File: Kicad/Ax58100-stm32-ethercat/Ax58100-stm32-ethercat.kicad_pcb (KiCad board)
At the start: 4 copper layers, 94.5 x 59.2 mm, 133 parts, among them J1 Conn_01x06_Pin, J10 Conn_01x02_Pin, J11 Stepper 2, J12 Serial usart1, J13 Stepper 1, J14 I2C bus2, J2 Encoder 1, J3 Conn_01x06_Pin, J4 Encoder 2, J5 Conn_01x06_Pin, J6 Encoder 4, J7 DAC1, J8 Encoder 3, J9 STLINK, SW1 SW PB, U1 AMS1117-1.2, U2 AX58100, U3 24LC32A, U4 STM32F407VGT6, U5 AMS1117-3.3, Y1 NXK25.000AE12F-KAB6-12, Y2 8 MHz

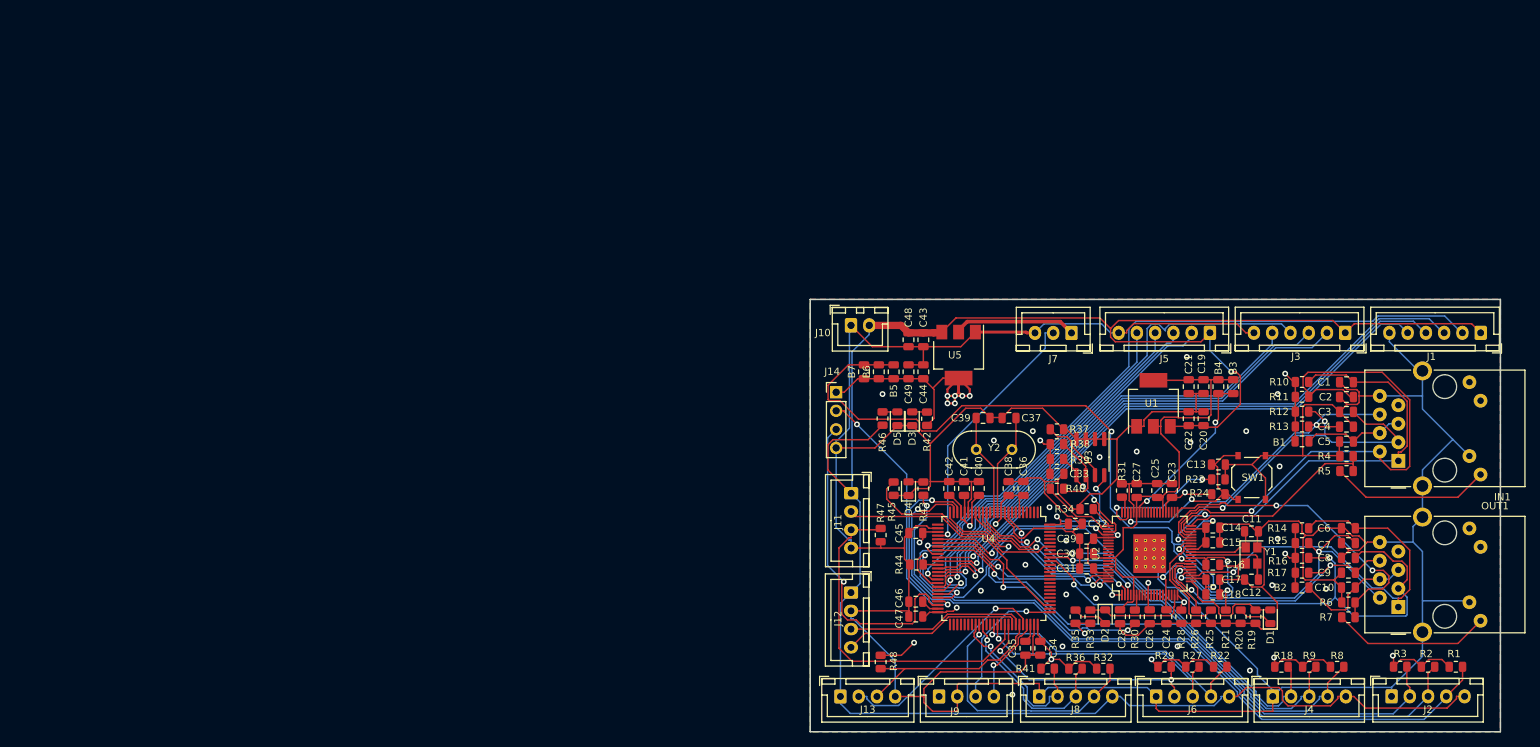
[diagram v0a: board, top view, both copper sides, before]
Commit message: First component placement
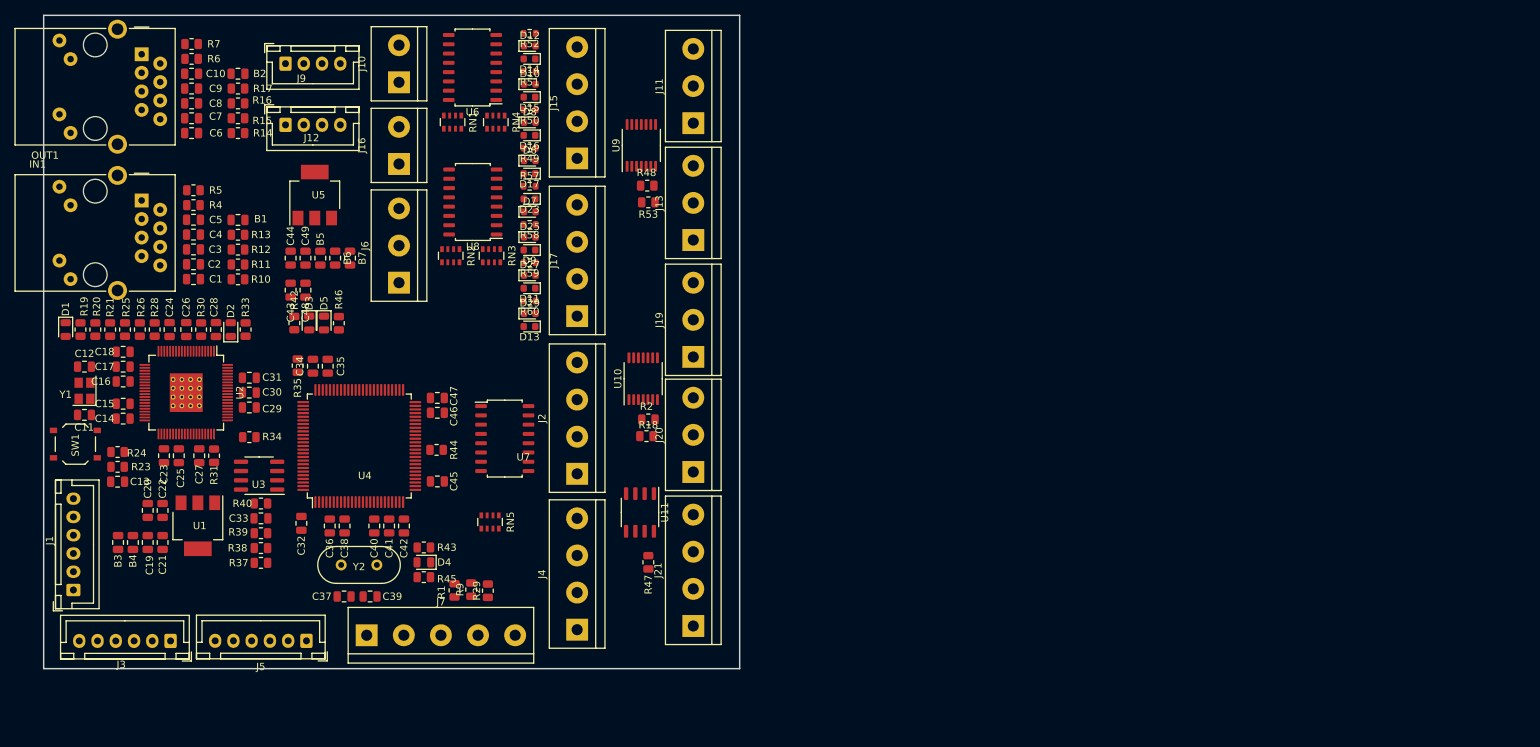
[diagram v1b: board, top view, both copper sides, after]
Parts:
- removed J14: I2C bus2, Connector_PinHeader_2.54mm:PinHeader_1x04_P2.54mm_Vertical
- removed J8: Encoder 3, Connector_JST:JST_XH_B5B-XH-A_1x05_P2.50mm_Vertical
- removed R22, R27, R3, R32, R36, R41, R8: 1k, Resistor_SMD:R_0805_2012Metric
- added D10: Yellow led, LED_SMD:LED_0603_1608Metric, F.Cu at (100.6, 34.3)
- added D11: Red led, LED_SMD:LED_0603_1608Metric, F.Cu at (100.5, 62.2)
- added D12: Yellow led, LED_SMD:LED_0603_1608Metric, F.Cu at (100.6, 29.1)
- added D13: Red led, LED_SMD:LED_0603_1608Metric, F.Cu at (100.5, 67.5)
- added D14: Red led, LED_SMD:LED_0603_1608Metric, F.Cu at (100.5, 30.8)
- added D15: Red led, LED_SMD:LED_0603_1608Metric, F.Cu at (100.5, 36.1)
- added D16: Red led, LED_SMD:LED_0603_1608Metric, F.Cu at (100.5, 41.3)
- added D17: Red led, LED_SMD:LED_0603_1608Metric, F.Cu at (100.5, 46.5)
- added D23: Yellow led, LED_SMD:LED_0603_1608Metric, F.Cu at (100.5, 50.0)
- added D25: Yellow led, LED_SMD:LED_0603_1608Metric, F.Cu at (100.6, 55.2)
- added D27: Yellow led, LED_SMD:LED_0603_1608Metric, F.Cu at (100.6, 60.5)
- added D29: Yellow led, LED_SMD:LED_0603_1608Metric, F.Cu at (100.6, 65.7)
- added D6: Yellow led, LED_SMD:LED_0603_1608Metric, F.Cu at (100.6, 44.8)
- added D7: Red led, LED_SMD:LED_0603_1608Metric, F.Cu at (100.6, 51.8)
- added D8: Yellow led, LED_SMD:LED_0603_1608Metric, F.Cu at (100.6, 39.5)
- added D9: Red led, LED_SMD:LED_0603_1608Metric, F.Cu at (100.5, 57.0)
- added J15: In1-4, TerminalBlock:TerminalBlock_bornier-4_P5.08mm, F.Cu at (107.0, 44.5)
- added J16: 24V Field, TerminalBlock:TerminalBlock_bornier-2_P5.08mm, F.Cu at (82.7, 45.2)
- added J17: In5-8, TerminalBlock:TerminalBlock_bornier-4_P5.08mm, F.Cu at (107.0, 66.0)
- added J19: Step3, TerminalBlock:TerminalBlock_bornier-3_P5.08mm, F.Cu at (122.9, 71.6)
- added J20: Step4, TerminalBlock:TerminalBlock_bornier-3_P5.08mm, F.Cu at (122.9, 87.4)
- added J21: THCAD, TerminalBlock:TerminalBlock_bornier-4_P5.08mm, F.Cu at (122.9, 108.5)
- added R49: 1k, Resistor_SMD:R_0603_1608Metric, F.Cu at (100.5, 43.0)
- added R50: 1k, Resistor_SMD:R_0603_1608Metric, F.Cu at (100.5, 37.8)
- added R51: 1k, Resistor_SMD:R_0603_1608Metric, F.Cu at (100.5, 32.6)
- added R52: 1k, Resistor_SMD:R_0603_1608Metric, F.Cu at (100.5, 27.3)
- added R53: 4.7k, Resistor_SMD:R_0805_2012Metric, F.Cu at (116.8, 50.5)
- added R57: 1k, Resistor_SMD:R_0603_1608Metric, F.Cu at (100.5, 48.3)
- added R58: 1k, Resistor_SMD:R_0603_1608Metric, F.Cu at (100.5, 53.5)
- added R59: 1k, Resistor_SMD:R_0603_1608Metric, F.Cu at (100.5, 58.7)
- added R60: 1k, Resistor_SMD:R_0603_1608Metric, F.Cu at (100.5, 64.0)
- added RN1: 40k, Resistor_SMD:R_Array_Convex_4x0603, F.Cu at (90.0, 39.5)
- added RN2: 40k, Resistor_SMD:R_Array_Convex_4x0603, F.Cu at (89.7, 57.8)
- added RN3: 1k, Resistor_SMD:R_Array_Convex_4x0603, F.Cu at (95.3, 57.8)
- added RN4: 1k, Resistor_SMD:R_Array_Convex_4x0603, F.Cu at (95.9, 39.5)
- added RN5: 330, Resistor_SMD:R_Array_Convex_4x0603, F.Cu at (95.1, 94.2)
- added U10: TXB0104PW, Package_SO:TSSOP-14_4.4x5mm_P0.65mm, F.Cu at (116.1, 74.6)
- added U11: MAX3485CSA/ESA, Package_SO:SO-8_3.9x4.9mm_P1.27mm, F.Cu at (115.6, 92.9)
- added U6: TLP292-4, Package_SO:SOIC-16_4.55x10.3mm_P1.27mm, F.Cu at (92.7, 32.0)
- added U7: TLP291-4, Package_SO:SOIC-16_4.55x10.3mm_P1.27mm, F.Cu at (97.1, 82.8)
- added U8: TLP292-4, Package_SO:SOIC-16_4.55x10.3mm_P1.27mm, F.Cu at (92.8, 50.4)
- added U9: TXB0104PW, Package_SO:TSSOP-14_4.4x5mm_P0.65mm, F.Cu at (115.8, 42.7)
- J1: value Conn_01x06_Pin -> Out_opt
- J10: value Conn_01x02_Pin -> 5V Power IN; footprint Connector_JST:JST_XH_B2B-XH-A_1x02_P2.50mm_Vertical -> TerminalBlock:TerminalBlock_bornier-2_P5.08mm
- J11: value Stepper 2 -> Step1; footprint Connector_JST:JST_XH_B4B-XH-A_1x04_P2.50mm_Vertical -> TerminalBlock:TerminalBlock_bornier-3_P5.08mm
- J13: value Stepper 1 -> Step2; footprint Connector_JST:JST_XH_B4B-XH-A_1x04_P2.50mm_Vertical -> TerminalBlock:TerminalBlock_bornier-3_P5.08mm
- J2: value Encoder 1 -> Output1-2; footprint Connector_JST:JST_XH_B5B-XH-A_1x05_P2.50mm_Vertical -> TerminalBlock:TerminalBlock_bornier-4_P5.08mm
- J3: value Conn_01x06_Pin -> In_opt1
- J4: value Encoder 2 -> Output3-4; footprint Connector_JST:JST_XH_B5B-XH-A_1x05_P2.50mm_Vertical -> TerminalBlock:TerminalBlock_bornier-4_P5.08mm
- J5: value Conn_01x06_Pin -> In_opt2
- J6: value Encoder 4 -> DAC; footprint Connector_JST:JST_XH_B5B-XH-A_1x05_P2.50mm_Vertical -> TerminalBlock:TerminalBlock_bornier-3_P5.08mm
- J7: value DAC1 -> Encoder; footprint Connector_JST:JST_XH_B3B-XH-A_1x03_P2.50mm_Vertical -> TerminalBlock:TerminalBlock_bornier-5_P5.08mm
- R18, R2: value 1k -> 4.7k
- R47: value NC -> 120
- R48: value NC -> 4.7k
- moved J1 195.8 mm to (38.1, 103.5), turned to 90 degrees
- moved OUT1 187.9 mm to (47.4, 30.2), turned to 90 degrees
- moved R7 176.7 mm to (54.3, 28.8), turned to 0 degrees
- moved IN1 175.7 mm to (47.4, 50.2), turned to 90 degrees
- moved R6 175.0 mm to (54.3, 30.8), turned to 0 degrees
- moved C10 173.3 mm to (54.3, 32.9), turned to 180 degrees
- moved C9 171.7 mm to (54.3, 34.9), turned to 180 degrees
- moved C8 170.1 mm to (54.3, 36.9), turned to 180 degrees
- moved D1 169.5 mm to (37.0, 67.9), turned to -90 degrees
- moved C7 168.7 mm to (54.3, 39.0), turned to 180 degrees
- moved C6 167.3 mm to (54.3, 41.0), turned to 180 degrees
- moved J3 166.2 mm to (51.4, 110.5)
- moved R19 165.6 mm to (39.0, 67.9), turned to -90 degrees
- moved R5 162.5 mm to (54.5, 48.8), turned to 0 degrees
- moved C12 162.4 mm to (39.6, 73.0), turned to 0 degrees
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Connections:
- J11 pad 1: +5V -> STEP1_DIR_OUT
- J11 pad 2: STEP2_DIR -> STEP1_STEP_OUT
- J11 pad 3: STEP2_STEP -> GND
- J13 pad 1: +5V -> STEP2_DIR_OUT
- J13 pad 2: STEP1_DIR -> STEP2_STEP_OUT
- J13 pad 3: STEP1_STEP -> GND
- J2 pad 1: GND -> Net-(J2-Pin_1)
- J2 pad 2: ENC1_Z -> Net-(J2-Pin_2)
- J2 pad 3: ENC1_B -> Net-(J2-Pin_3)
- J2 pad 4: ENC1_A -> Net-(J2-Pin_4)
- J4 pad 1: GND -> Net-(J4-Pin_1)
- J4 pad 2: ENC2_Z -> Net-(J4-Pin_2)
- J4 pad 3: ENC2_B -> Net-(J4-Pin_3)
- J4 pad 4: ENC2_A -> Net-(J4-Pin_4)
- J6 pad 1: GND -> +3.3V
- J6 pad 2: ENC4_Z -> DAC1
- J6 pad 3: ENC4_B -> GND
- J7 pad 1: +3.3V -> +5V
- J7 pad 2: DAC1 -> ENC_A
- J7 pad 3: GND -> ENC_B
- R1 pad 1: ENC1_A -> ENC_A
- R1 pad 2: +3.3V -> +5V
- R18 pad 1: ENC2_Z -> GND
- R18 pad 2: +3.3V -> STEP4_STEP
- R2 pad 1: ENC1_B -> GND
- R2 pad 2: +3.3V -> STEP3_STEP
- R29 pad 1: ENC4_Z -> ENC_Z
- R29 pad 2: +3.3V -> +5V
- R47 pad 1: STEP2_STEP -> Net-(J21-Pin_2)
- R47 pad 2: GND -> Net-(J21-Pin_3)
- R48 pad 1: STEP1_STEP -> GND
- R48 pad 2: GND -> STEP1_STEP
- R9 pad 1: ENC2_B -> ENC_B
- R9 pad 2: +3.3V -> +5V
- U4 pad 23: ENC1_A -> ENC_A
- U4 pad 24: ENC1_B -> ENC_B
- U4 pad 25: ENC1_Z -> THCAD_CTR
- U4 pad 26: unconnected-(U4-PA3-Pad26) -> ENC_Z
- U4 pad 3: unconnected-(U4-PE4-Pad3) -> STEP4_DIR
- U4 pad 4: unconnected-(U4-PE5-Pad4) -> STEP4_STEP
- U4 pad 47: I2C2_SCL -> unconnected-(U4-PB10-Pad47)
- U4 pad 48: I2C2_SDA -> unconnected-(U4-PB11-Pad48)
- U4 pad 58: ENC3_Z -> STEP3_DIR
- U4 pad 59: ENC3_A -> STEP3_STEP
- U4 pad 60: ENC3_B -> unconnected-(U4-PD13-Pad60)
- U4 pad 63: ENC4_A -> unconnected-(U4-PC6-Pad63)
- U4 pad 64: ENC4_B -> unconnected-(U4-PC7-Pad64)
- U4 pad 65: unconnected-(U4-PC8-Pad65) -> STEP2_DIR
- U4 pad 67: ENC4_Z -> unconnected-(U4-PA8-Pad67)
- U4 pad 78: STEP2_DIR -> unconnected-(U4-PC10-Pad78)
- U4 pad 90: ENC2_A -> unconnected-(U4-PB4-Pad90)
- U4 pad 91: ENC2_B -> unconnected-(U4-PB5-Pad91)
- U4 pad 92: ENC2_Z -> unconnected-(U4-PB6-Pad92)
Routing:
- net GND: track 682.4 -> 0.00 mm, vias 24 -> 0
- net +5V: track 289.8 -> 0.00 mm, vias 1 -> 0
- net +3.3V: track 209.3 -> 0.00 mm, vias 23 -> 0
- net +3.3VA: track 109.3 -> 0.00 mm, vias 4 -> 0
- net ENC1_A: track 105.7 -> 0.00 mm, vias 1 -> 0
- net ENC1_B: track 100.3 -> 0.00 mm, vias 1 -> 0
- net +1V2: track 97.9 -> 0.00 mm, vias 2 -> 0
- net IO1: track 93.0 -> 0.00 mm, vias 1 -> 0
- net ENC1_Z: track 86.5 -> 0.00 mm, vias 1 -> 0
- net IO2: track 83.8 -> 0.00 mm, vias 1 -> 0
- net IO3: track 81.9 -> 0.00 mm, vias 1 -> 0
- net IO4: track 80.7 -> 0.00 mm, vias 1 -> 0
- net IO8: track 77.5 -> 0.00 mm, vias 1 -> 0
- net P0_TXON: track 75.4 -> 0.00 mm, vias 1 -> 0
- net IO5: track 72.0 -> 0.00 mm, vias 1 -> 0
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- removed copper zone on In2.Cu, net +3.3V
- removed copper zone on B.Cu, net GND
- removed copper zone on F.Cu, net GND
- removed copper zone on In1.Cu, net GND
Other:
- board size 94.5 x 59.2 mm -> 95.3 x 89.4 mm
